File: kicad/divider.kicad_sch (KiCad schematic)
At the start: 28 parts, among them J40 SPI, Q17 2N3904, Q18 2N3904, Q2 2N3904, Q3 2N3904, Q4 2N3904, Q5 2N3904, Q6 2N3904, Q7 2N3904, Q8 2N3904, U12 ATtiny24A-P

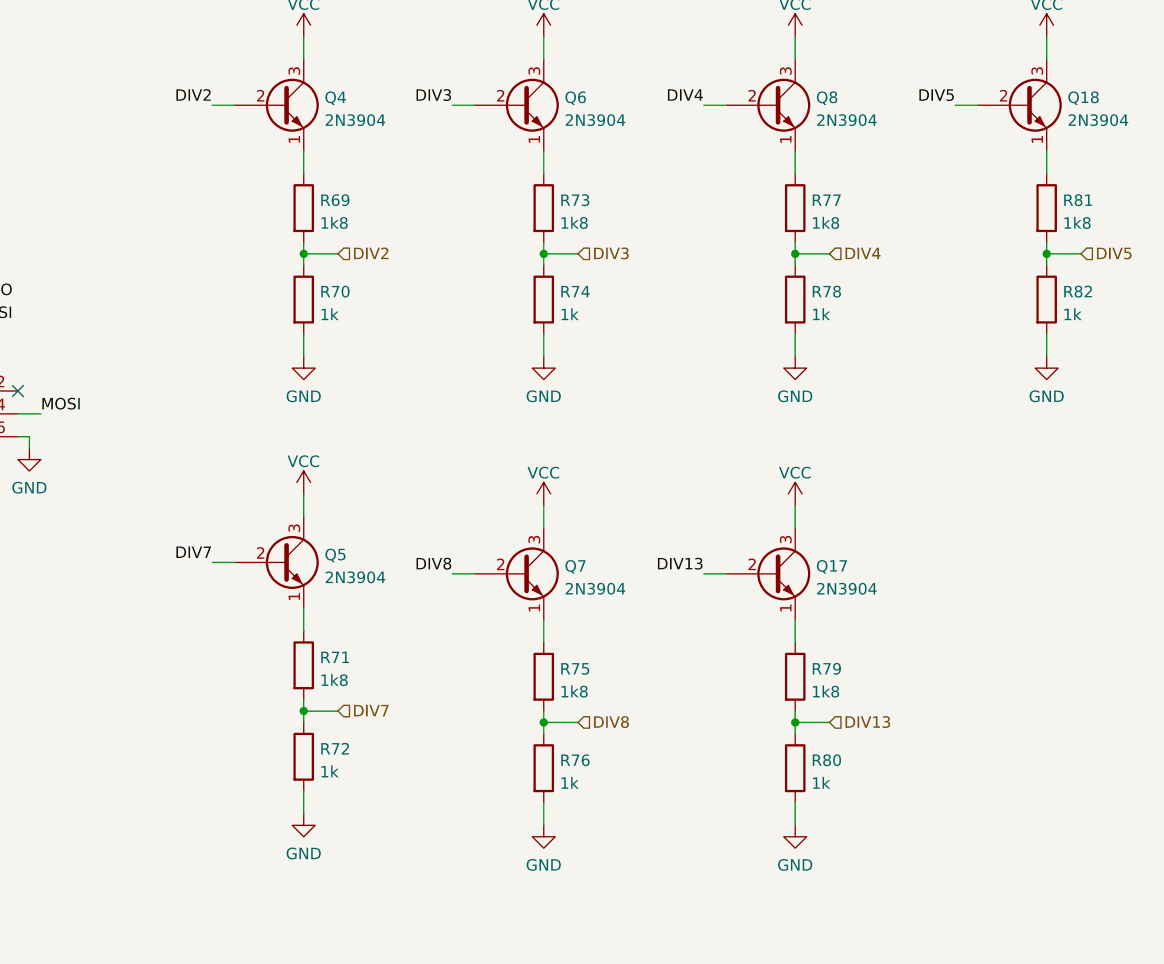
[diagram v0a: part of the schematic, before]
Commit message: Finished most recent redesign
probably still needs fixing though
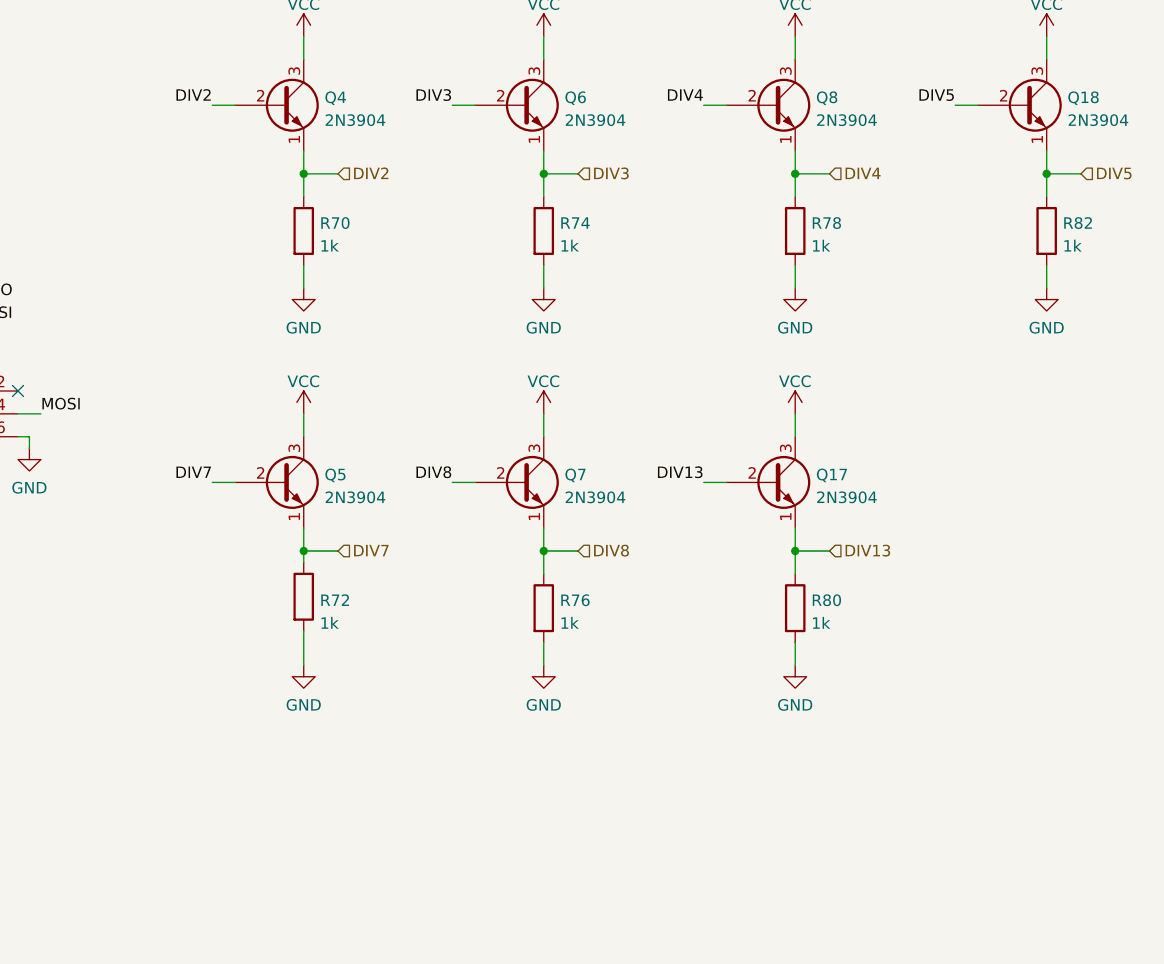
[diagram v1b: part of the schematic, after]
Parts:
- removed R69, R71, R73, R75, R77, R79, R81: 1k8, rumblesan-standard-parts:R_Axial_DIN0207_L6.3mm_D2.5mm_P10.16mm_Horizontal, symbol rumblesan-standard-parts:R
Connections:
- net DIV13: now also Q17.1 (E)
- net DIV2: now also Q4.1 (E)
- net DIV3: now also Q6.1 (E)
- net DIV4: now also Q8.1 (E)
- net DIV5: now also Q18.1 (E)
- net DIV7: now also Q5.1 (E)
- net DIV8: now also Q7.1 (E)
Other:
- moved on the sheet: Q17, Q5, Q7, R70, R72, R74, R76, R78, R80, R82
